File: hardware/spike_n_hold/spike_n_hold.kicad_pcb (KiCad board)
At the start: 2 copper layers, 63 x 110.5 mm, 61 parts, among them J1 input_trigger_2, J2 input_trigger_1, J3 to_solenoid_2, J4 to_solenoid_1, J5 Conn_01x02, J6 Conn_01x02, J7 Conn_01x02, Q1 MJH11021G, Q2 MJH11021G, Q3 MPSA42, Q4 MPSA42, Q5 MPSA42, Q6 MPSA42, Q7 MJH11022G, Q8 MJH11022G, Q9 IRFZ24NPBF, U1 LM555xM, U2 LM555xM, U3 LM555xM

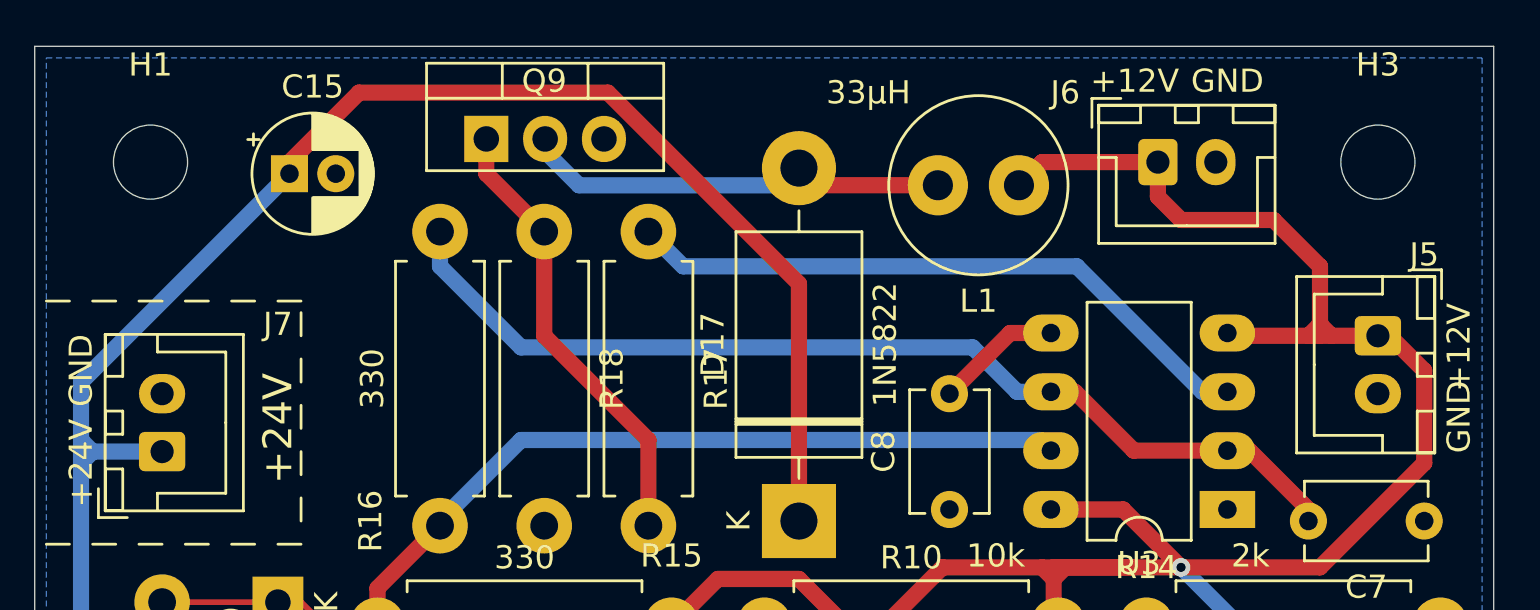
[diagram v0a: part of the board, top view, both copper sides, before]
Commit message: Update board and add gerbers
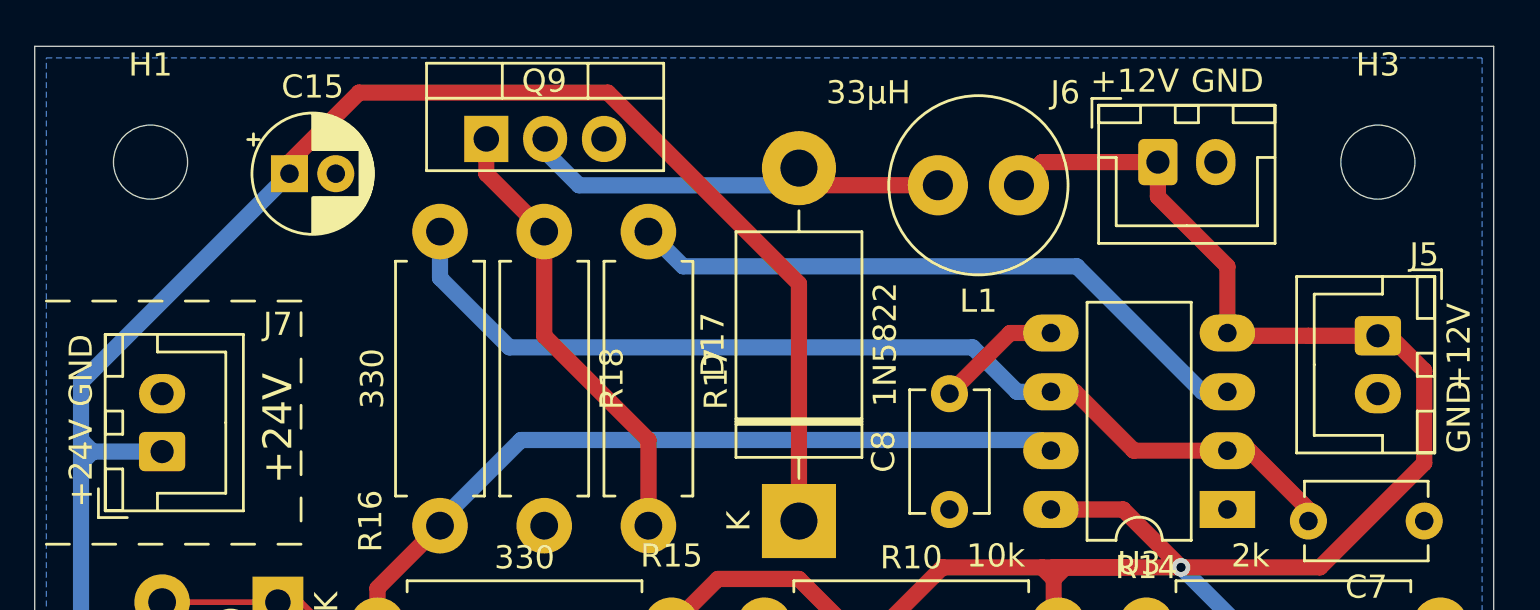
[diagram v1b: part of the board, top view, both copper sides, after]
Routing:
- net +12V: track 217.5 -> 212.0 mm
